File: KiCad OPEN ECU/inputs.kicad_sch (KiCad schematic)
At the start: 41 parts, among them J3 EBC05DRXN, SW1 219-2MSTR, U10 SP720, U13 LMV324LIDT, U18 KP234

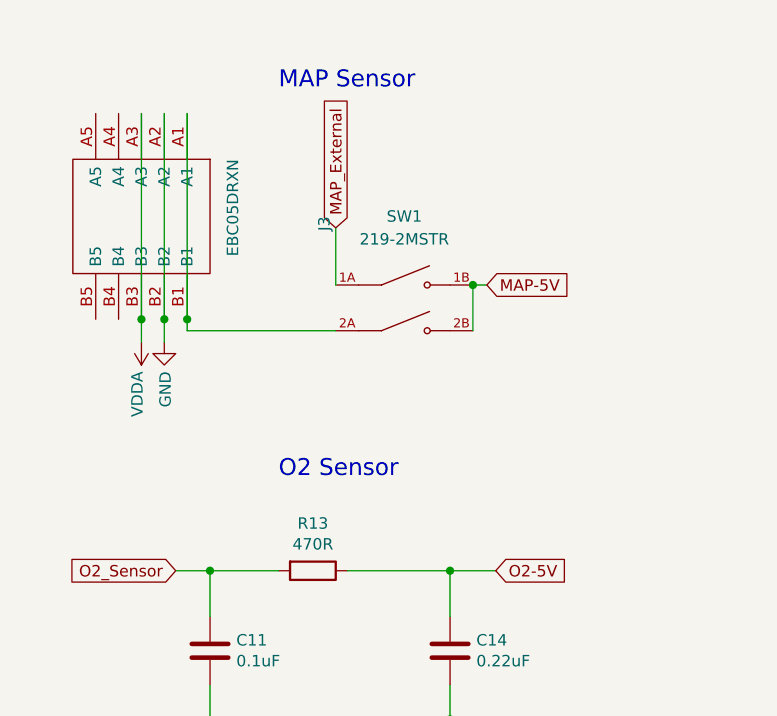
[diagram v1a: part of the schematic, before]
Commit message: Add files via upload
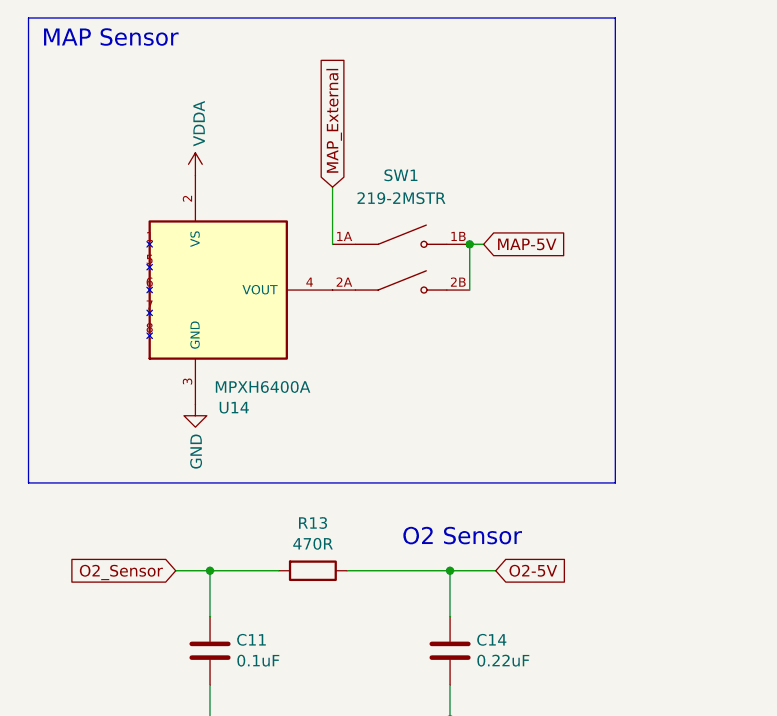
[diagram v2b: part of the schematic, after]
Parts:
- removed J3: EBC05DRXN, Misc:EBC05DRXN, symbol Misc:EBC05DRXN
- added U14: MPXH6400A, AeonLabs_Sensors:NXP MAP Sensor, symbol AeonLabs_Sensors:MPXH6400A_MAP_Sensor
- C13, C18, C19, C21, C22, C23: footprint Capacitor_SMD:C_0805_2012Metric -> Capacitor_SMD:C_0603_1608Metric
- R12: footprint Resistor_SMD:R_0603_1608Metric_Pad1.05x0.95mm_HandSolder -> Resistor_SMD:R_0603_1608Metric
- R15, R17, R18, R19, R21, R22: footprint Resistor_SMD:R_0805_2012Metric -> Resistor_SMD:R_0603_1608Metric
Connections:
- net GND: now also U14.3 (GND)
- net VDDA: now also U14.2 (VS)
- net at SW1.2A: now also U14.4 (VOUT)
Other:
- moved on the sheet: SW1
